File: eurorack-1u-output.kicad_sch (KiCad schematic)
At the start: 18 parts, among them J1 Eurorack_Power_10pin_Unshroud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, U1 TL072, U2 TL072

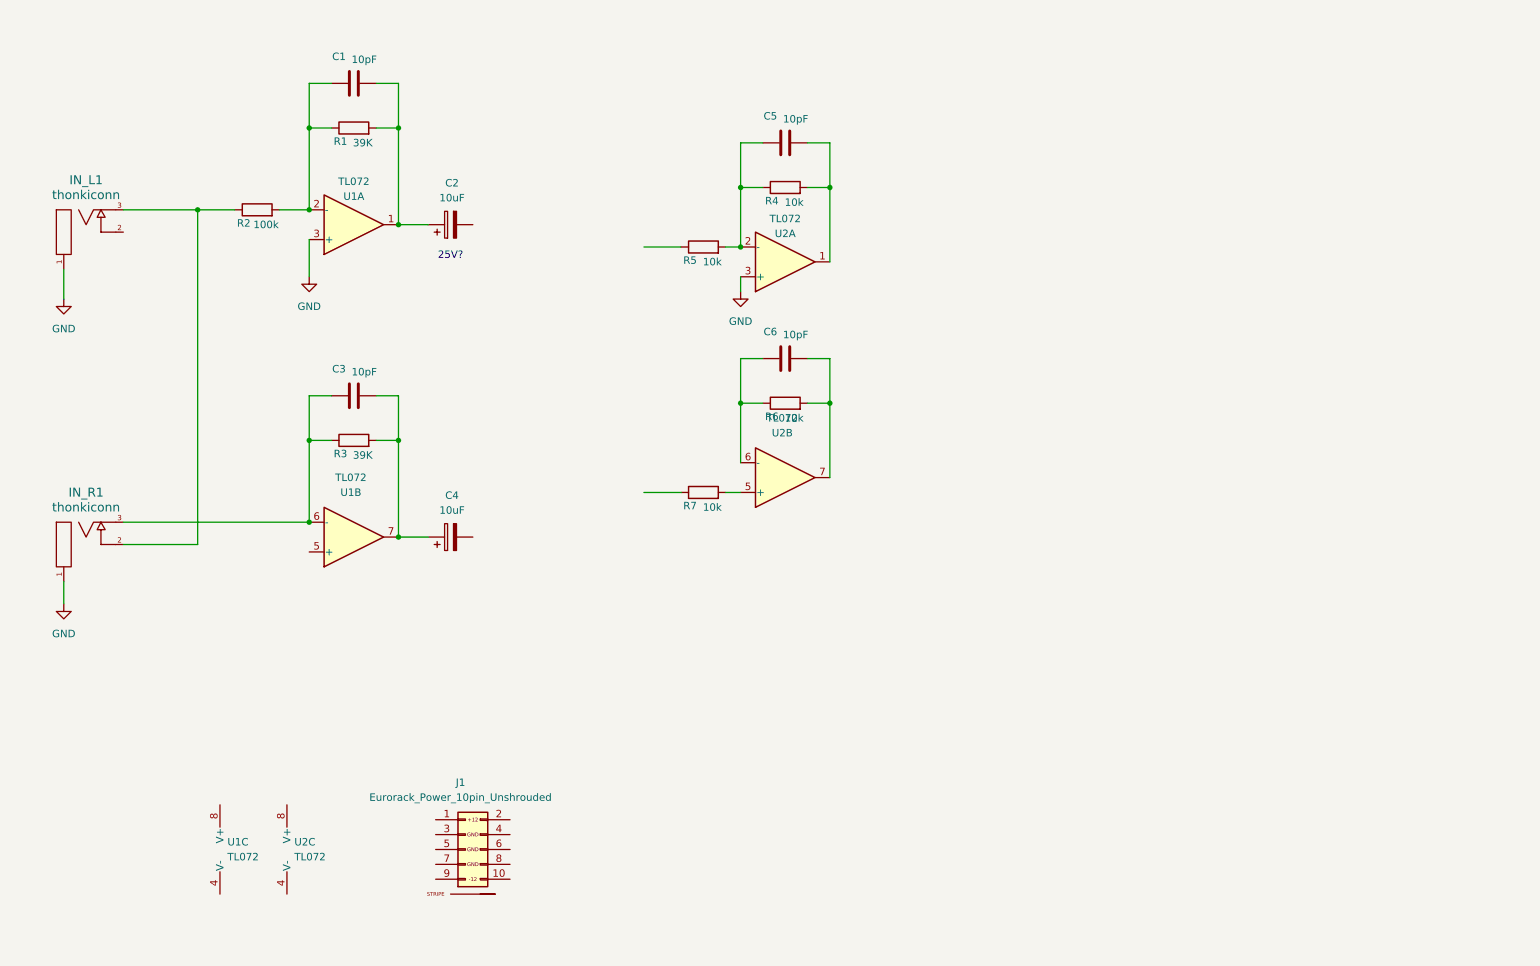
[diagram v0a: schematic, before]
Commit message: some progress
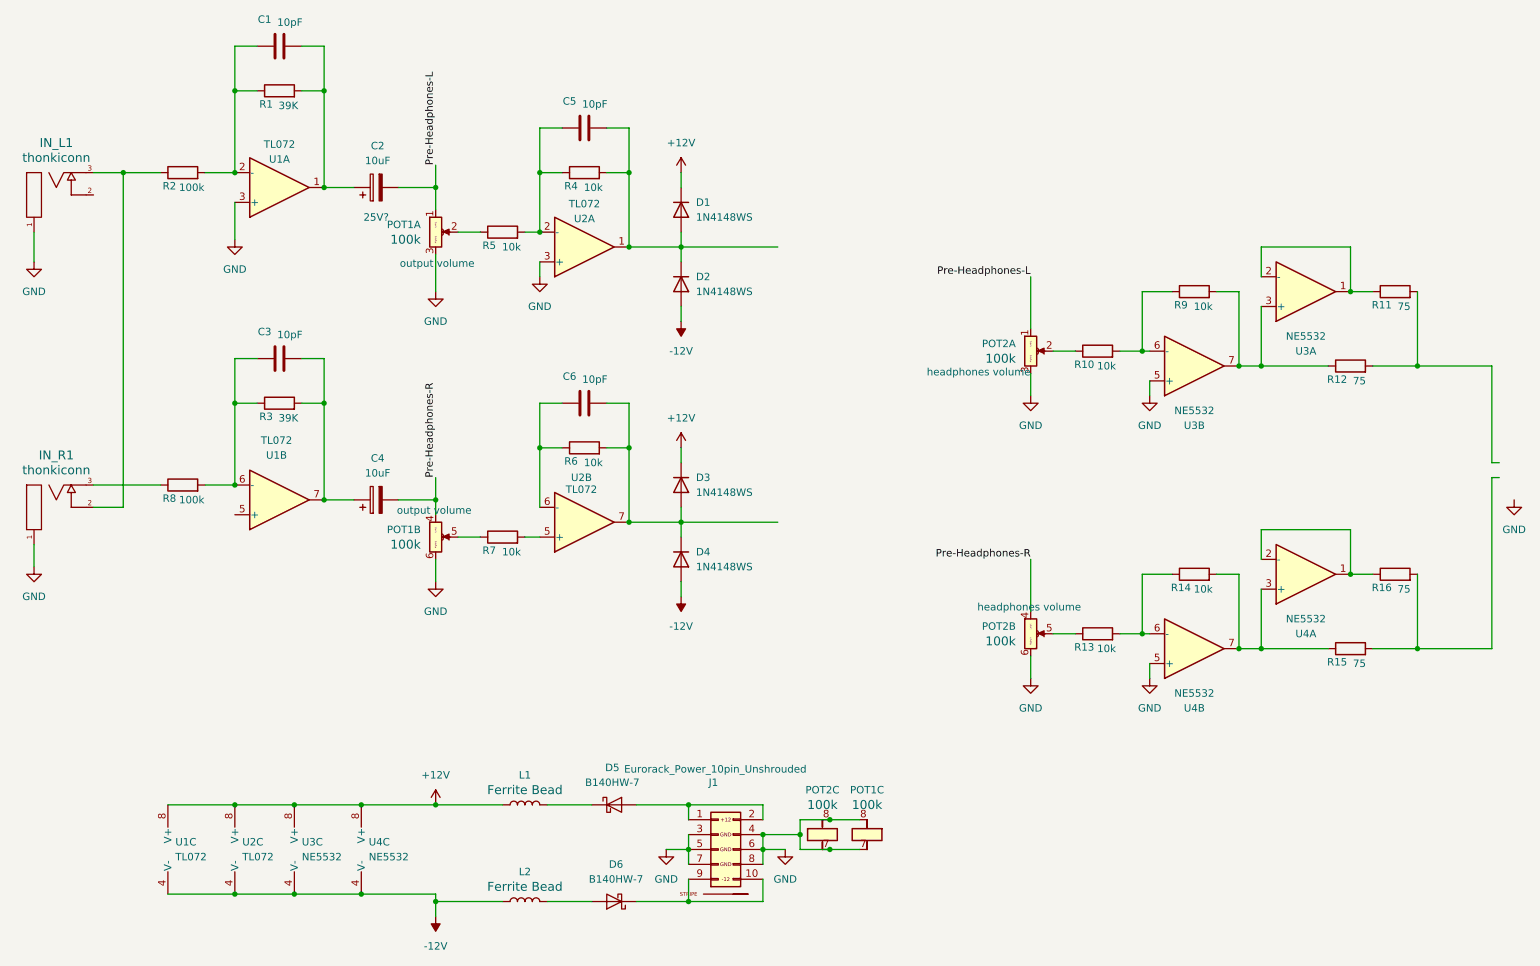
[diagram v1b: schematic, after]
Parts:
- added D1, D2, D3, D4: 1N4148WS, Diode_SMD:D_SOD-323, symbol Diode:1N4148WS
- added D5, D6: B140HW-7, Diode_SMD:D_SOD-123, symbol PCM_4ms_Diode:B140HW-7
- added L1, L2: FerriteBead_0603_1.5A, Inductor_SMD:L_0603_1608Metric, symbol PCM_4ms_Inductor:FerriteBead_0603_1.5A
- added POT1: output volume, PCM_4ms_Potentiometer:Potentiometer_Alps_RK09L_Double_Vertical, symbol aa-sampozki:9mm_alphastereo_100k_Knurled_Lined
- added POT2: headphones volume, PCM_4ms_Potentiometer:Potentiometer_Alps_RK09L_Double_Vertical, symbol aa-sampozki:9mm_alphastereo_100k_Knurled_Lined
- added R10, R13, R14, R9: 10k, Resistor_SMD:R_0603_1608Metric, symbol Device:R
- added R11, R12, R15, R16: 75, Resistor_SMD:R_0603_1608Metric, symbol Device:R
- added R8: 100k, Resistor_SMD:R_0603_1608Metric, symbol Device:R
- added U3, U4: NE5532, Package_SO:SOIC-8_3.9x4.9mm_P1.27mm, symbol Amplifier_Operational:NE5532
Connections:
- net GND: now also J1.3 (GND), J1.4 (GND), J1.5 (GND), J1.6 (GND), J1.7 (GND), J1.8 (GND), POT1.3 (Right), POT1.6 (Right), POT1.7 (Tab1), POT1.8 (Tab2), POT2.3 (Right), POT2.6 (Right), POT2.7 (Tab1), POT2.8 (Tab2), U3.5 (+), U4.5 (+)
- net -12V: now reaches U2.4 (V-)
- net -12V: now also U1.4 (V-), D2.2 (A), D4.2 (A), L2.1, U3.4 (V-), U4.4 (V-)
- net +12V: now reaches U2.8 (V+)
- net +12V: now also U1.8 (V+), D1.1 (K), D3.1 (K), L1.1, U3.8 (V+), U4.8 (V+)
- net at C3.1, R3.1, U1.6 (-): now also R8.2; no longer IN_R1.3 (SIG)
- net at R7.1: now also POT1.5 (Center)
- net at J1.1 (+12V): now also J1.2 (+12V), D5.2 (A)
- net at J1.10 (-12V): now also J1.9 (-12V), D6.1 (K)
- net Pre-Headphones-R: now reaches C4.2
- net Pre-Headphones-R: now also POT1.4 (Left), POT2.4 (Left)
- net at R5.1: now also POT1.2 (Center)
- net at C5.2, R4.2, U2.1: now also D1.2 (A), D2.1 (K)
- net at C6.2, R6.2, U2.7: now also D3.2 (A), D4.1 (K)
- net Pre-Headphones-L: now reaches C2.2
- net Pre-Headphones-L: now also POT1.1 (Left), POT2.1 (Left)
- new net: IN_R1.3 (SIG), R8.1
- new net: D5.1 (K), L1.2
- new net: R12.1, R9.2, U3.3 (+), U3.7
- new net: R11.2, R12.2
- new net: R11.1, U3.1, U3.2 (-)
- new net: R16.1, U4.1, U4.2 (-)
- new net: R14.2, R15.1, U4.3 (+), U4.7
- new net: POT2.2 (Center), R10.1
- new net: R10.2, R9.1, U3.6 (-)
- new net: R15.2, R16.2
- new net: R13.2, R14.1, U4.6 (-)
- new net: POT2.5 (Center), R13.1
- new net: D6.2 (A), L2.2
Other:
- moved on the sheet: C1, C2, C3, C4, C5, C6, IN_L1, IN_R1, J1, R1, R2, R3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
